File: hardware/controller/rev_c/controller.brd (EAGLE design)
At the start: 68.1 x 80 mm, 106 parts, among them J1 DM3AT-SF-PEJM5, J10 SOLDERJUMPERTRACE, J11 SOLDERJUMPERTRACE, J12 SOLDERJUMPERTRACE, J14 TC2030-JLINK-L, J15 TC2030-JLINK-L, J16 U.FL-R-SMT, J2 MICRO_USB_B_HIROSE_ZX62R-B-5P, J3 MICRO_USB_B_HIROSE_ZX62R-B-5P, J4 MODULE_CONTROLLER, J9 SOLDERJUMPERTRACE, Q1 DMN32D2LDF, SW1 B3U-1000P, SW2 B3U-1000P, SW3 B3U-1000P, SW4 B3U-1000P, SW5 SIP3240X, SW6 SIP3240X, SW7 SIP3240X, U1 FM25CLXXB-DG, U10 TXS0108EVQFN20, U2 FTDI234XD, U3 NCP301LSN30, U4 NCP301LSN30, U5 RXM-GPS-RM-T, U6 SAM4LC8BA, U7 SAM4LC8BA, U8 SN74LVC1G125DBVR, U9 TS3USB30E, X1 16MHz, X2 16MHz

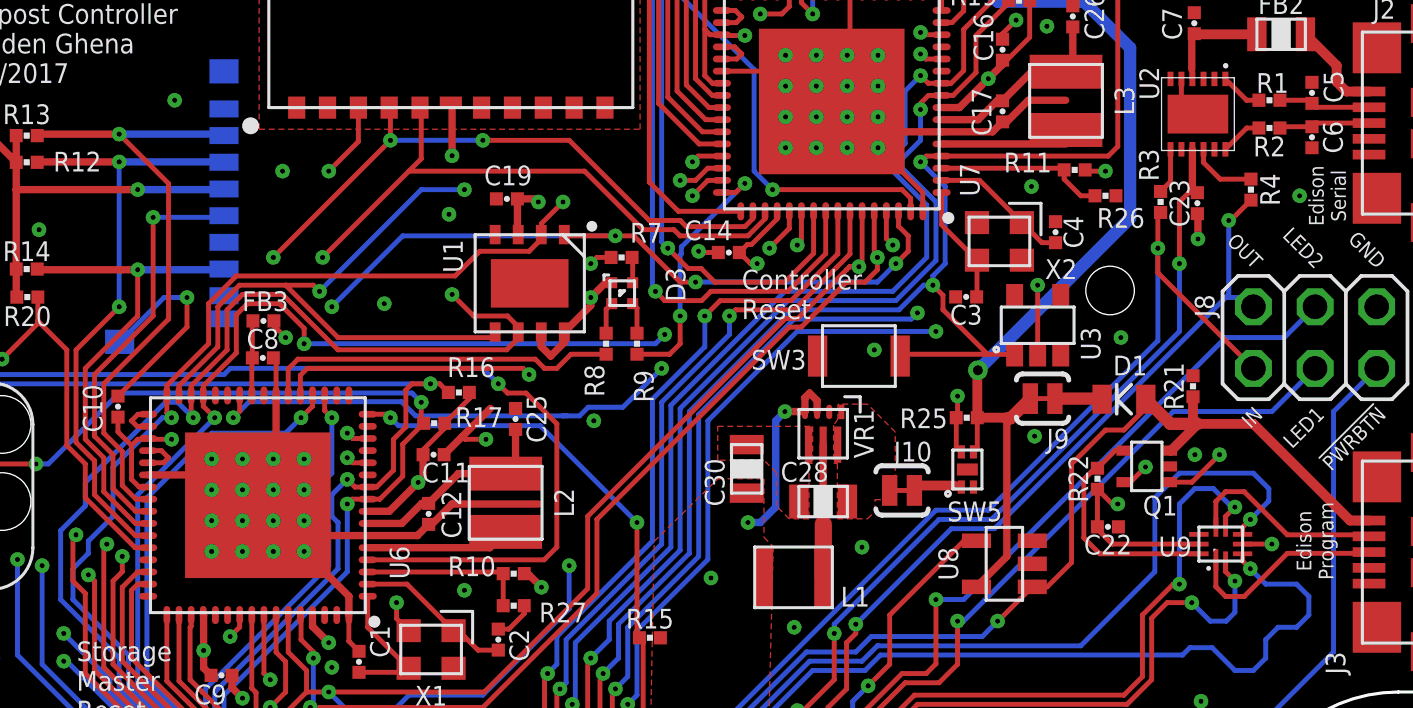
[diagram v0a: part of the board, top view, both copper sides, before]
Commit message: Added updates from Pat & Josh
Pulldown on 1v8 output enable
PPS connection to storage master

Did NOT add module in/out pins for the edison
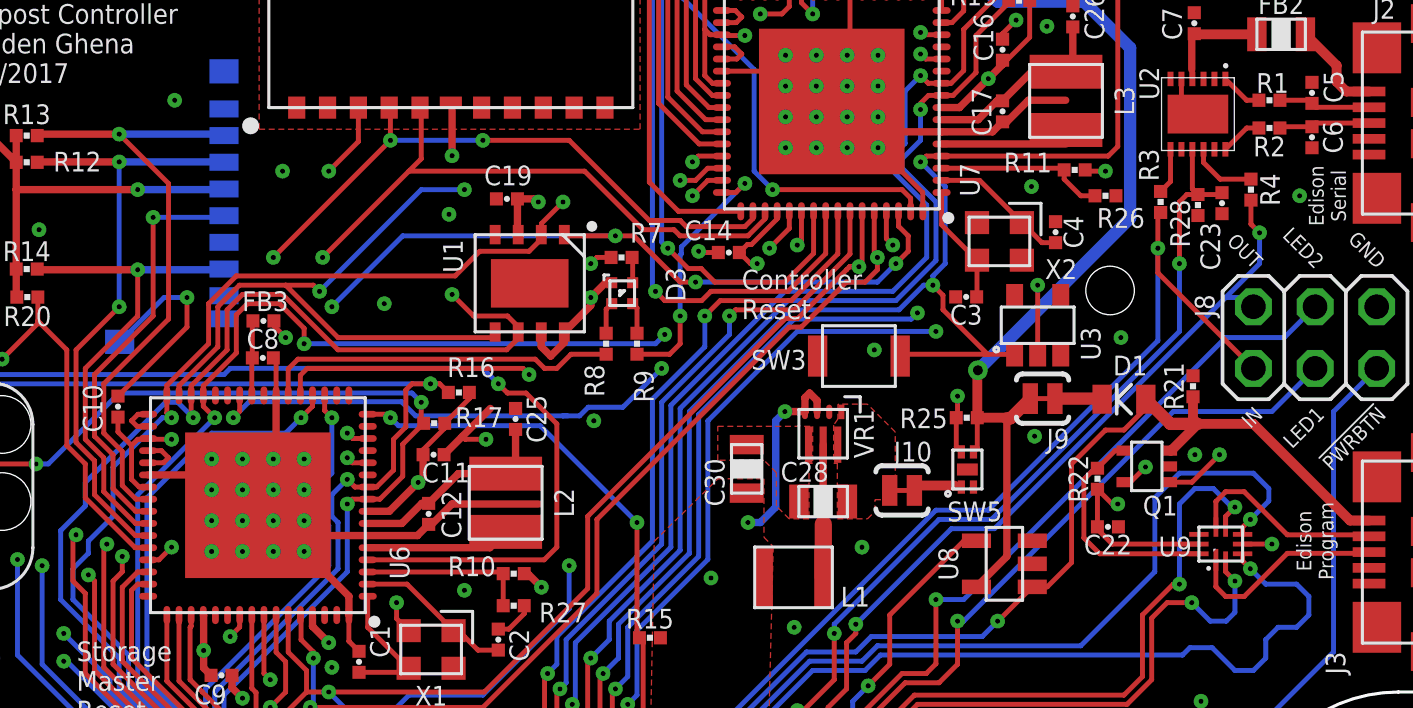
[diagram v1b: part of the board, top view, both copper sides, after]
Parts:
- added R28: 100kΩ, passives:0402_RES
- moved C23 1.02 mm to (23.9, 5.54)
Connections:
- net GND: now also R28.2
- net PPS: now also U6.45
- net VCC_LINUX_1V8: now also R28.1
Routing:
- net PPS: track 76.8 -> 98.8 mm, vias 3 -> 4
- net VCC_LINUX_1V8: track 84.0 -> 85.1 mm
- net GND: track 201.9 -> 200.9 mm, vias 79 -> 78
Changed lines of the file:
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@@
 <attribute name="NAME" x="19.1516" y="-8.9408" size="0.8128" layer="25" font="vector" ratio="12" align="bottom-center"/>
 </element>
-<element name="C23" library="passives" package="0402_CAP" value="100nF" x="22.836" y="5.5372" smashed="yes" rot="R270">
-<attribute name="DIGIKEY" value="490-10777-1-ND" x="22.836" y="4.2672" size="1.778" layer="27" rot="R270" display="off"/>
-<attribute name="NAME" x="21.693" y="5.5372" size="0.8128" layer="25" font="vector" ratio="12" rot="R270" align="bottom-center"/>
+<element name="C23" library="passives" package="0402_CAP" value="100nF" x="23.852" y="5.5372" smashed="yes" rot="R270">
+<attribute name="DIGIKEY" value="490-10777-1-ND" x="23.852" y="4.2672" size="1.778" layer="27" rot="R270" display="off"/>
+<attribute name="NAME" x="22.963" y="3.7592" size="0.8128" layer="25" font="vector" ratio="12" rot="R270" align="bottom-center"/>
 </element>
 <element name="C7" library="passives" package="0402_CAP" value="10nF" x="22.709" y="12.954" smashed="yes" rot="R90">
@@
 <attribute name="NAME" x="-21.336" y="-22.86" size="0.8128" layer="25" font="vector" ratio="12" rot="R180" align="bottom-center"/>
 <attribute name="VALUE" x="-21.336" y="-18.796" size="1.016" layer="27" font="vector" ratio="12" align="bottom-center"/>
+</element>
+<element name="R28" library="passives" package="0402_RES" value="100kΩ" x="22.86" y="5.461" smashed="yes" rot="R270">
+<attribute name="DIGIKEY" value="1276-3432-1-ND" x="22.86" y="4.953" size="1.778" layer="27" rot="R270" display="off"/>
+<attribute name="NAME" x="21.717" y="4.699" size="0.8128" layer="25" font="vector" ratio="12" rot="R270" align="bottom-center"/>
+<attribute name="VALUE" x="21.463" y="5.461" size="1.016" layer="27" font="vector" ratio="12" rot="R270" align="bottom-center"/>
 </element>
 </elements>
@@
 <wire x1="22.86" y1="9.2075" x2="22.18" y2="9.8875" width="0.2032" layer="1"/>
 <wire x1="22.18" y1="9.8875" x2="22.18" y2="10.6575" width="0.2032" layer="1"/>
-<wire x1="22.836" y1="5.10413125" x2="22.86" y2="5.08013125" width="0.3048" layer="1"/>
-<wire x1="22.86" y1="5.08013125" x2="22.86" y2="4.064" width="0.3048" layer="1"/>
-<via x="22.86" y="4.064" extent="1-16" drill="0.2032"/>
 <wire x1="-20.32" y1="21.795" x2="-20.32" y2="24.638" width="0.3048" layer="1"/>
 <via x="-20.32" y="24.638" extent="1-16" drill="0.2032"/>
@@
 <wire x1="3.09753125" y1="3.5052" x2="2.3368" y2="3.5052" width="0.2032" layer="1"/>
 <wire x1="2.3368" y1="3.5052" x2="2.286" y2="3.556" width="0.2032" layer="1"/>
+<contactref element="R28" pad="2"/>
 </signal>
 <signal name="PPS">
@@
 <wire x1="-11.7348" y1="8.0772" x2="-12.954" y2="6.858" width="0.2032" layer="1"/>
 <via x="-12.954" y="6.858" extent="1-16" drill="0.2032"/>
-<wire x1="-12.954" y1="6.858" x2="0.254" y2="6.858" width="0.2032" layer="2"/>
+<wire x1="0.254" y1="6.858" x2="-12.954" y2="6.858" width="0.2032" layer="2"/>
 <via x="2.032" y="7.239" extent="1-16" drill="0.2032"/>
 <wire x1="-3.048" y1="-9.398" x2="-3.048" y2="-6.604" width="0.2032" layer="2"/>
@@
 <wire x1="2.032" y1="7.239" x2="0.635" y2="7.239" width="0.2032" layer="2"/>
 <wire x1="0.635" y1="7.239" x2="0.254" y2="6.858" width="0.2032" layer="2"/>
+<contactref element="U6" pad="45"/>
+<wire x1="-12.954" y1="6.858" x2="-12.954" y2="3.83826875" width="0.2032" layer="2"/>
+<wire x1="-12.2682" y1="-1.7018" x2="-12.192" y2="-1.778" width="0.2032" layer="2"/>
+<wire x1="-12.954" y1="3.83826875" x2="-12.2682" y2="3.15246875" width="0.2032" layer="2"/>
+<wire x1="-12.2682" y1="3.15246875" x2="-12.2682" y2="-1.7018" width="0.2032" layer="2"/>
+<wire x1="-12.192" y1="-1.778" x2="-13.1572" y2="-2.7432" width="0.2032" layer="2"/>
+<wire x1="-13.1572" y1="-2.7432" x2="-14.32846875" y2="-2.7432" width="0.2032" layer="2"/>
+<wire x1="-15.44606875" y1="-3.8608" x2="-17.78" y2="-3.8608" width="0.2032" layer="2"/>
+<wire x1="-17.78" y1="-3.8608" x2="-19.431" y2="-5.5118" width="0.2032" layer="2"/>
+<wire x1="-14.32846875" y1="-2.7432" x2="-15.44606875" y2="-3.8608" width="0.2032" layer="2"/>
+<via x="-19.431" y="-8.636" extent="1-16" drill="0.2032"/>
+<wire x1="-19.431" y1="-5.5118" x2="-19.431" y2="-8.636" width="0.2032" layer="2"/>
+<wire x1="-20.4" y1="-9.1588" x2="-19.9538" y2="-9.1588" width="0.2032" layer="1"/>
+<wire x1="-19.9538" y1="-9.1588" x2="-19.431" y2="-8.636" width="0.2032" layer="1"/>
 </signal>
 <signal name="N$1">
@@
 <via x="3.556" y="-20.828" extent="1-16" drill="0.2032"/>
 <via x="8.763" y="-11.811" extent="1-16" drill="0.2032"/>
-<via x="24.13" y="4.826" extent="1-16" drill="0.2032"/>
 <wire x1="8.763" y1="-11.811" x2="12.7" y2="-7.874" width="0.2032" layer="16"/>
 <wire x1="12.7" y1="-7.874" x2="14.478" y2="-7.874" width="0.2032" layer="16"/>
 <contactref element="J8" pad="5"/>
 <wire x1="14.478" y1="-7.874" x2="24.003" y2="1.651" width="0.2032" layer="16"/>
-<wire x1="24.003" y1="1.651" x2="24.13" y2="1.778" width="0.2032" layer="16"/>
-<wire x1="24.13" y1="1.778" x2="24.13" y2="4.826" width="0.2032" layer="16"/>
 <wire x1="25.146" y1="1.27" x2="24.765" y2="1.651" width="0.2032" layer="16"/>
 <wire x1="24.765" y1="1.651" x2="24.003" y2="1.651" width="0.2032" layer="16"/>
@@
 <wire x1="8.382" y1="-12.573" x2="8.763" y2="-12.192" width="0.2032" layer="1"/>
 <wire x1="8.763" y1="-12.192" x2="8.763" y2="-11.811" width="0.2032" layer="1"/>
-<wire x1="25.0444" y1="5.66293125" x2="24.20746875" y2="4.826" width="0.2032" layer="1"/>
-<wire x1="24.20746875" y1="4.826" x2="24.13" y2="4.826" width="0.2032" layer="1"/>
+<wire x1="25.4" y1="3.048" x2="25.4" y2="4.318" width="0.2032" layer="16"/>
+<via x="25.4" y="4.318" extent="1-16" drill="0.2032"/>
+<wire x1="25.4" y1="4.318" x2="25.0444" y2="4.6736" width="0.2032" layer="1"/>
+<wire x1="25.0444" y1="4.6736" x2="25.0444" y2="5.66293125" width="0.2032" layer="1"/>
+<wire x1="24.003" y1="1.651" x2="25.4" y2="3.048" width="0.2032" layer="16"/>
 </signal>
 <signal name="N$28">
@@
 <contactref element="C24" pad="2"/>
 <contactref element="J7" pad="14"/>
-<wire x1="22.63" y1="7.7575" x2="22.63" y2="6.17626875" width="0.3048" layer="1"/>
-<wire x1="22.63" y1="6.17626875" x2="22.836" y2="5.97026875" width="0.3048" layer="1"/>
 <wire x1="-10.1985" y1="-27.1754" x2="-10.1985" y2="-28.64993125" width="0.2032" layer="1"/>
 <wire x1="-10.1985" y1="-28.64993125" x2="-10.14643125" y2="-28.702" width="0.2032" layer="1"/>
@@
 <via x="22.098" y="3.048" extent="1-16" drill="0.2032"/>
 <wire x1="22.098" y1="3.048" x2="22.098" y2="5.588" width="0.2032" layer="1"/>
-<wire x1="22.098" y1="5.588" x2="22.48026875" y2="5.97026875" width="0.2032" layer="1"/>
-<wire x1="22.48026875" y1="5.97026875" x2="22.836" y2="5.97026875" width="0.2032" layer="1"/>
 <wire x1="6.35" y1="-17.931609375" x2="6.35" y2="-15.367" width="0.3048" layer="15"/>
 <wire x1="6.35" y1="-17.931609375" x2="4.977609375" y2="-19.304" width="0.3048" layer="15"/>
@@
 <wire x1="7.874" y1="-14.097" x2="6.604" y2="-15.367" width="0.2032" layer="1"/>
 <wire x1="6.604" y1="-15.367" x2="6.35" y2="-15.367" width="0.2032" layer="1"/>
+<contactref element="R28" pad="1"/>
+<wire x1="22.40406875" y1="5.89406875" x2="22.098" y2="5.588" width="0.2032" layer="1"/>
+<wire x1="22.40406875" y1="5.89406875" x2="22.86" y2="5.89406875" width="0.2032" layer="1"/>
+<wire x1="22.63" y1="7.7575" x2="22.63" y2="6.12406875" width="0.2032" layer="1"/>
+<wire x1="22.63" y1="6.12406875" x2="22.86" y2="5.89406875" width="0.2032" layer="1"/>
+<wire x1="22.86" y1="5.89406875" x2="23.7758" y2="5.89406875" width="0.2032" layer="1"/>
+<wire x1="23.7758" y1="5.89406875" x2="23.852" y2="5.97026875" width="0.2032" layer="1"/>
 </signal>
 <signal name="N$34">

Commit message: Actual version C sent to fab
Mistakenly forgot OE pull down and PPS to storage master
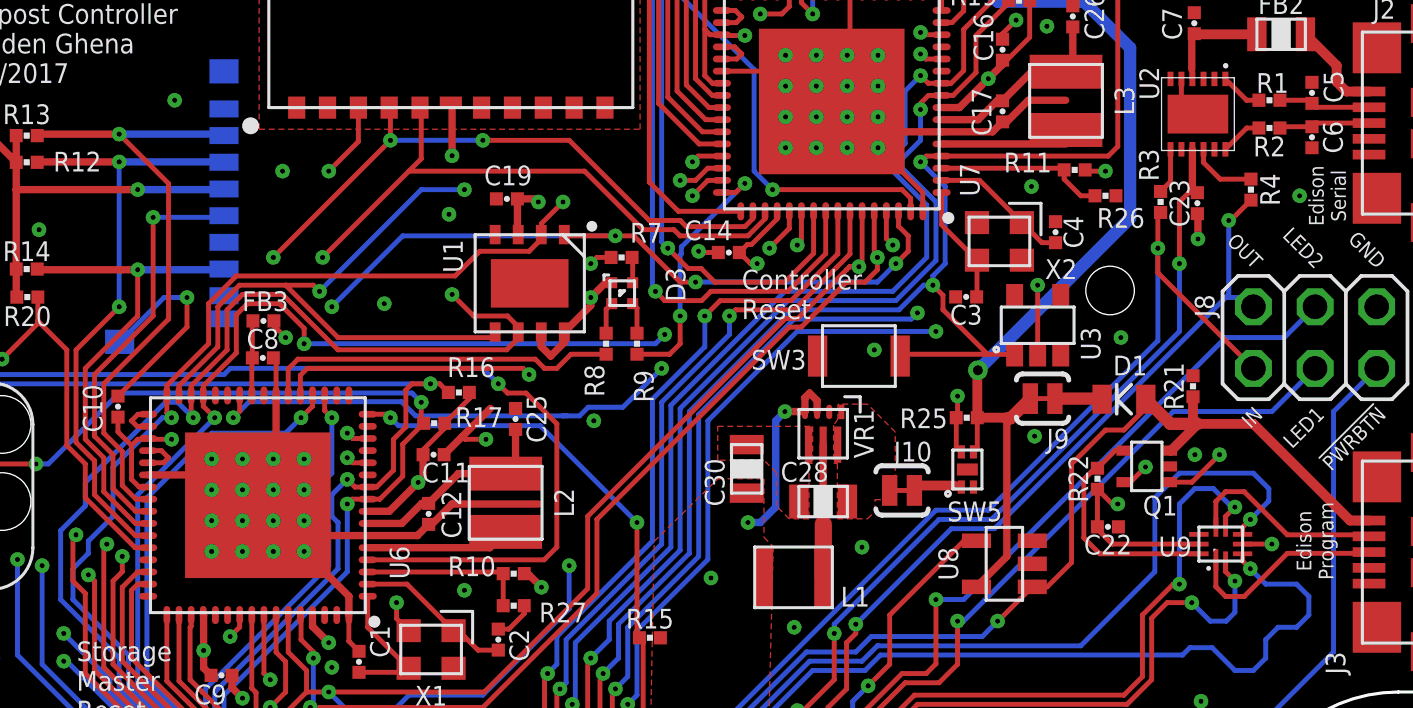
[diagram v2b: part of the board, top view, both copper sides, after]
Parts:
- removed R28: 100kΩ, passives:0402_RES
- moved C23 1.02 mm to (22.8, 5.54)
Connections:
- net GND: no longer R28.2
- net PPS: no longer U6.45
- net VCC_LINUX_1V8: no longer R28.1
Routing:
- net PPS: track 98.8 -> 76.8 mm, vias 4 -> 3
- net VCC_LINUX_1V8: track 85.1 -> 84.0 mm
- net GND: track 200.9 -> 201.9 mm, vias 78 -> 79
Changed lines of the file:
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@@
 <attribute name="NAME" x="19.1516" y="-8.9408" size="0.8128" layer="25" font="vector" ratio="12" align="bottom-center"/>
 </element>
-<element name="C23" library="passives" package="0402_CAP" value="100nF" x="23.852" y="5.5372" smashed="yes" rot="R270">
-<attribute name="DIGIKEY" value="490-10777-1-ND" x="23.852" y="4.2672" size="1.778" layer="27" rot="R270" display="off"/>
-<attribute name="NAME" x="22.963" y="3.7592" size="0.8128" layer="25" font="vector" ratio="12" rot="R270" align="bottom-center"/>
+<element name="C23" library="passives" package="0402_CAP" value="100nF" x="22.836" y="5.5372" smashed="yes" rot="R270">
+<attribute name="DIGIKEY" value="490-10777-1-ND" x="22.836" y="4.2672" size="1.778" layer="27" rot="R270" display="off"/>
+<attribute name="NAME" x="21.693" y="5.5372" size="0.8128" layer="25" font="vector" ratio="12" rot="R270" align="bottom-center"/>
 </element>
 <element name="C7" library="passives" package="0402_CAP" value="10nF" x="22.709" y="12.954" smashed="yes" rot="R90">
@@
 <attribute name="NAME" x="-21.336" y="-22.86" size="0.8128" layer="25" font="vector" ratio="12" rot="R180" align="bottom-center"/>
 <attribute name="VALUE" x="-21.336" y="-18.796" size="1.016" layer="27" font="vector" ratio="12" align="bottom-center"/>
-</element>
-<element name="R28" library="passives" package="0402_RES" value="100kΩ" x="22.86" y="5.461" smashed="yes" rot="R270">
-<attribute name="DIGIKEY" value="1276-3432-1-ND" x="22.86" y="4.953" size="1.778" layer="27" rot="R270" display="off"/>
-<attribute name="NAME" x="21.717" y="4.699" size="0.8128" layer="25" font="vector" ratio="12" rot="R270" align="bottom-center"/>
-<attribute name="VALUE" x="21.463" y="5.461" size="1.016" layer="27" font="vector" ratio="12" rot="R270" align="bottom-center"/>
 </element>
 </elements>
@@
 <wire x1="22.86" y1="9.2075" x2="22.18" y2="9.8875" width="0.2032" layer="1"/>
 <wire x1="22.18" y1="9.8875" x2="22.18" y2="10.6575" width="0.2032" layer="1"/>
+<wire x1="22.836" y1="5.10413125" x2="22.86" y2="5.08013125" width="0.3048" layer="1"/>
+<wire x1="22.86" y1="5.08013125" x2="22.86" y2="4.064" width="0.3048" layer="1"/>
+<via x="22.86" y="4.064" extent="1-16" drill="0.2032"/>
 <wire x1="-20.32" y1="21.795" x2="-20.32" y2="24.638" width="0.3048" layer="1"/>
 <via x="-20.32" y="24.638" extent="1-16" drill="0.2032"/>
@@
 <wire x1="3.09753125" y1="3.5052" x2="2.3368" y2="3.5052" width="0.2032" layer="1"/>
 <wire x1="2.3368" y1="3.5052" x2="2.286" y2="3.556" width="0.2032" layer="1"/>
-<contactref element="R28" pad="2"/>
 </signal>
 <signal name="PPS">
@@
 <wire x1="-11.7348" y1="8.0772" x2="-12.954" y2="6.858" width="0.2032" layer="1"/>
 <via x="-12.954" y="6.858" extent="1-16" drill="0.2032"/>
-<wire x1="0.254" y1="6.858" x2="-12.954" y2="6.858" width="0.2032" layer="2"/>
+<wire x1="-12.954" y1="6.858" x2="0.254" y2="6.858" width="0.2032" layer="2"/>
 <via x="2.032" y="7.239" extent="1-16" drill="0.2032"/>
 <wire x1="-3.048" y1="-9.398" x2="-3.048" y2="-6.604" width="0.2032" layer="2"/>
@@
 <wire x1="2.032" y1="7.239" x2="0.635" y2="7.239" width="0.2032" layer="2"/>
 <wire x1="0.635" y1="7.239" x2="0.254" y2="6.858" width="0.2032" layer="2"/>
-<contactref element="U6" pad="45"/>
-<wire x1="-12.954" y1="6.858" x2="-12.954" y2="3.83826875" width="0.2032" layer="2"/>
-<wire x1="-12.2682" y1="-1.7018" x2="-12.192" y2="-1.778" width="0.2032" layer="2"/>
-<wire x1="-12.954" y1="3.83826875" x2="-12.2682" y2="3.15246875" width="0.2032" layer="2"/>
-<wire x1="-12.2682" y1="3.15246875" x2="-12.2682" y2="-1.7018" width="0.2032" layer="2"/>
-<wire x1="-12.192" y1="-1.778" x2="-13.1572" y2="-2.7432" width="0.2032" layer="2"/>
-<wire x1="-13.1572" y1="-2.7432" x2="-14.32846875" y2="-2.7432" width="0.2032" layer="2"/>
-<wire x1="-15.44606875" y1="-3.8608" x2="-17.78" y2="-3.8608" width="0.2032" layer="2"/>
-<wire x1="-17.78" y1="-3.8608" x2="-19.431" y2="-5.5118" width="0.2032" layer="2"/>
-<wire x1="-14.32846875" y1="-2.7432" x2="-15.44606875" y2="-3.8608" width="0.2032" layer="2"/>
-<via x="-19.431" y="-8.636" extent="1-16" drill="0.2032"/>
-<wire x1="-19.431" y1="-5.5118" x2="-19.431" y2="-8.636" width="0.2032" layer="2"/>
-<wire x1="-20.4" y1="-9.1588" x2="-19.9538" y2="-9.1588" width="0.2032" layer="1"/>
-<wire x1="-19.9538" y1="-9.1588" x2="-19.431" y2="-8.636" width="0.2032" layer="1"/>
 </signal>
 <signal name="N$1">
@@
 <via x="3.556" y="-20.828" extent="1-16" drill="0.2032"/>
 <via x="8.763" y="-11.811" extent="1-16" drill="0.2032"/>
+<via x="24.13" y="4.826" extent="1-16" drill="0.2032"/>
 <wire x1="8.763" y1="-11.811" x2="12.7" y2="-7.874" width="0.2032" layer="16"/>
 <wire x1="12.7" y1="-7.874" x2="14.478" y2="-7.874" width="0.2032" layer="16"/>
 <contactref element="J8" pad="5"/>
 <wire x1="14.478" y1="-7.874" x2="24.003" y2="1.651" width="0.2032" layer="16"/>
+<wire x1="24.003" y1="1.651" x2="24.13" y2="1.778" width="0.2032" layer="16"/>
+<wire x1="24.13" y1="1.778" x2="24.13" y2="4.826" width="0.2032" layer="16"/>
 <wire x1="25.146" y1="1.27" x2="24.765" y2="1.651" width="0.2032" layer="16"/>
 <wire x1="24.765" y1="1.651" x2="24.003" y2="1.651" width="0.2032" layer="16"/>
@@
 <wire x1="8.382" y1="-12.573" x2="8.763" y2="-12.192" width="0.2032" layer="1"/>
 <wire x1="8.763" y1="-12.192" x2="8.763" y2="-11.811" width="0.2032" layer="1"/>
-<wire x1="25.4" y1="3.048" x2="25.4" y2="4.318" width="0.2032" layer="16"/>
-<via x="25.4" y="4.318" extent="1-16" drill="0.2032"/>
-<wire x1="25.4" y1="4.318" x2="25.0444" y2="4.6736" width="0.2032" layer="1"/>
-<wire x1="25.0444" y1="4.6736" x2="25.0444" y2="5.66293125" width="0.2032" layer="1"/>
-<wire x1="24.003" y1="1.651" x2="25.4" y2="3.048" width="0.2032" layer="16"/>
+<wire x1="25.0444" y1="5.66293125" x2="24.20746875" y2="4.826" width="0.2032" layer="1"/>
+<wire x1="24.20746875" y1="4.826" x2="24.13" y2="4.826" width="0.2032" layer="1"/>
 </signal>
 <signal name="N$28">
@@
 <contactref element="C24" pad="2"/>
 <contactref element="J7" pad="14"/>
+<wire x1="22.63" y1="7.7575" x2="22.63" y2="6.17626875" width="0.3048" layer="1"/>
+<wire x1="22.63" y1="6.17626875" x2="22.836" y2="5.97026875" width="0.3048" layer="1"/>
 <wire x1="-10.1985" y1="-27.1754" x2="-10.1985" y2="-28.64993125" width="0.2032" layer="1"/>
 <wire x1="-10.1985" y1="-28.64993125" x2="-10.14643125" y2="-28.702" width="0.2032" layer="1"/>
@@
 <via x="22.098" y="3.048" extent="1-16" drill="0.2032"/>
 <wire x1="22.098" y1="3.048" x2="22.098" y2="5.588" width="0.2032" layer="1"/>
+<wire x1="22.098" y1="5.588" x2="22.48026875" y2="5.97026875" width="0.2032" layer="1"/>
+<wire x1="22.48026875" y1="5.97026875" x2="22.836" y2="5.97026875" width="0.2032" layer="1"/>
 <wire x1="6.35" y1="-17.931609375" x2="6.35" y2="-15.367" width="0.3048" layer="15"/>
 <wire x1="6.35" y1="-17.931609375" x2="4.977609375" y2="-19.304" width="0.3048" layer="15"/>
@@
 <wire x1="7.874" y1="-14.097" x2="6.604" y2="-15.367" width="0.2032" layer="1"/>
 <wire x1="6.604" y1="-15.367" x2="6.35" y2="-15.367" width="0.2032" layer="1"/>
-<contactref element="R28" pad="1"/>
-<wire x1="22.40406875" y1="5.89406875" x2="22.098" y2="5.588" width="0.2032" layer="1"/>
-<wire x1="22.40406875" y1="5.89406875" x2="22.86" y2="5.89406875" width="0.2032" layer="1"/>
-<wire x1="22.63" y1="7.7575" x2="22.63" y2="6.12406875" width="0.2032" layer="1"/>
-<wire x1="22.63" y1="6.12406875" x2="22.86" y2="5.89406875" width="0.2032" layer="1"/>
-<wire x1="22.86" y1="5.89406875" x2="23.7758" y2="5.89406875" width="0.2032" layer="1"/>
-<wire x1="23.7758" y1="5.89406875" x2="23.852" y2="5.97026875" width="0.2032" layer="1"/>
 </signal>
 <signal name="N$34">
